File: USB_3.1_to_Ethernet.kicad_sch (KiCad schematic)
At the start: 5 parts, among them J1 RJ45_JK0654219, U1 LAN7801_9JX, U2 93LC56B_SN, U3 KSZ9031RNXCC, Y1 C3E-8.000-18-3030-R

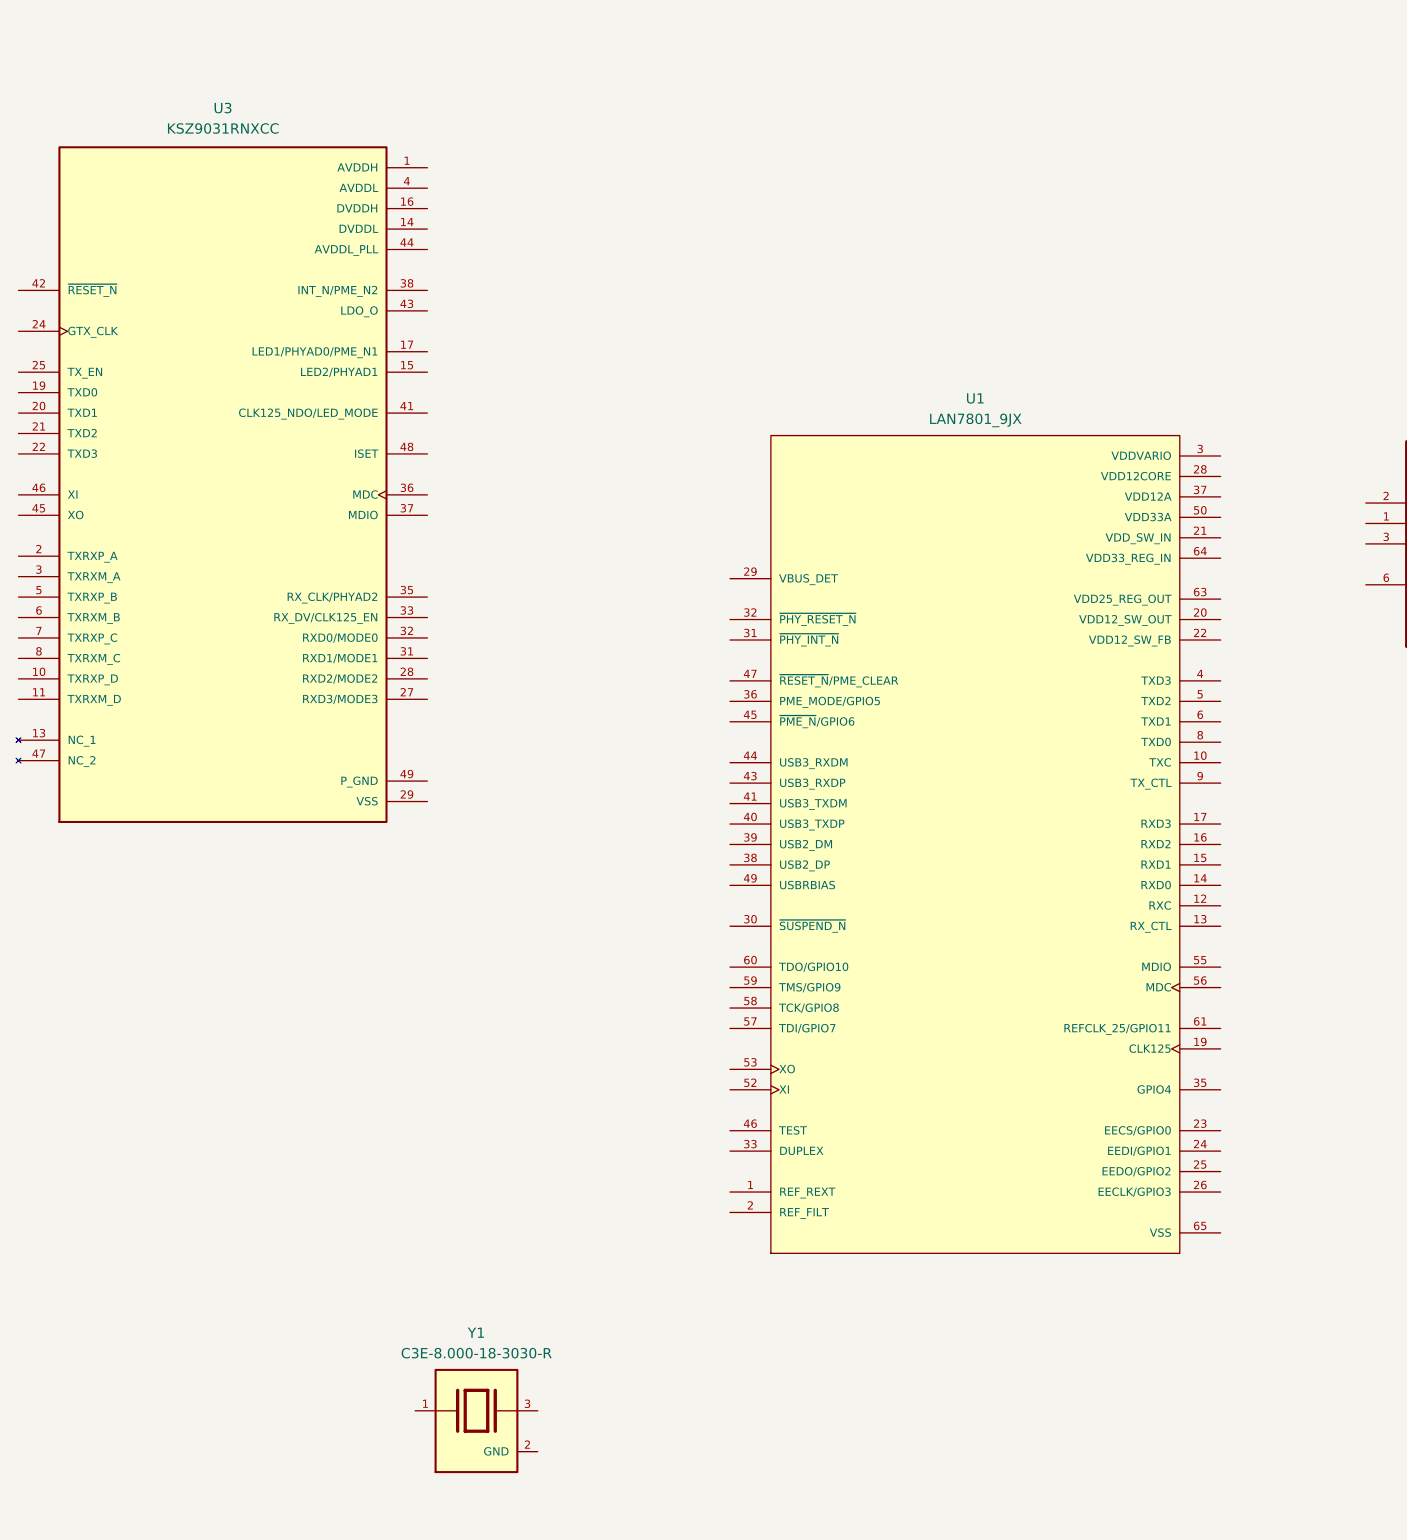
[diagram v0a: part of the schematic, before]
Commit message: power section added and power conections made
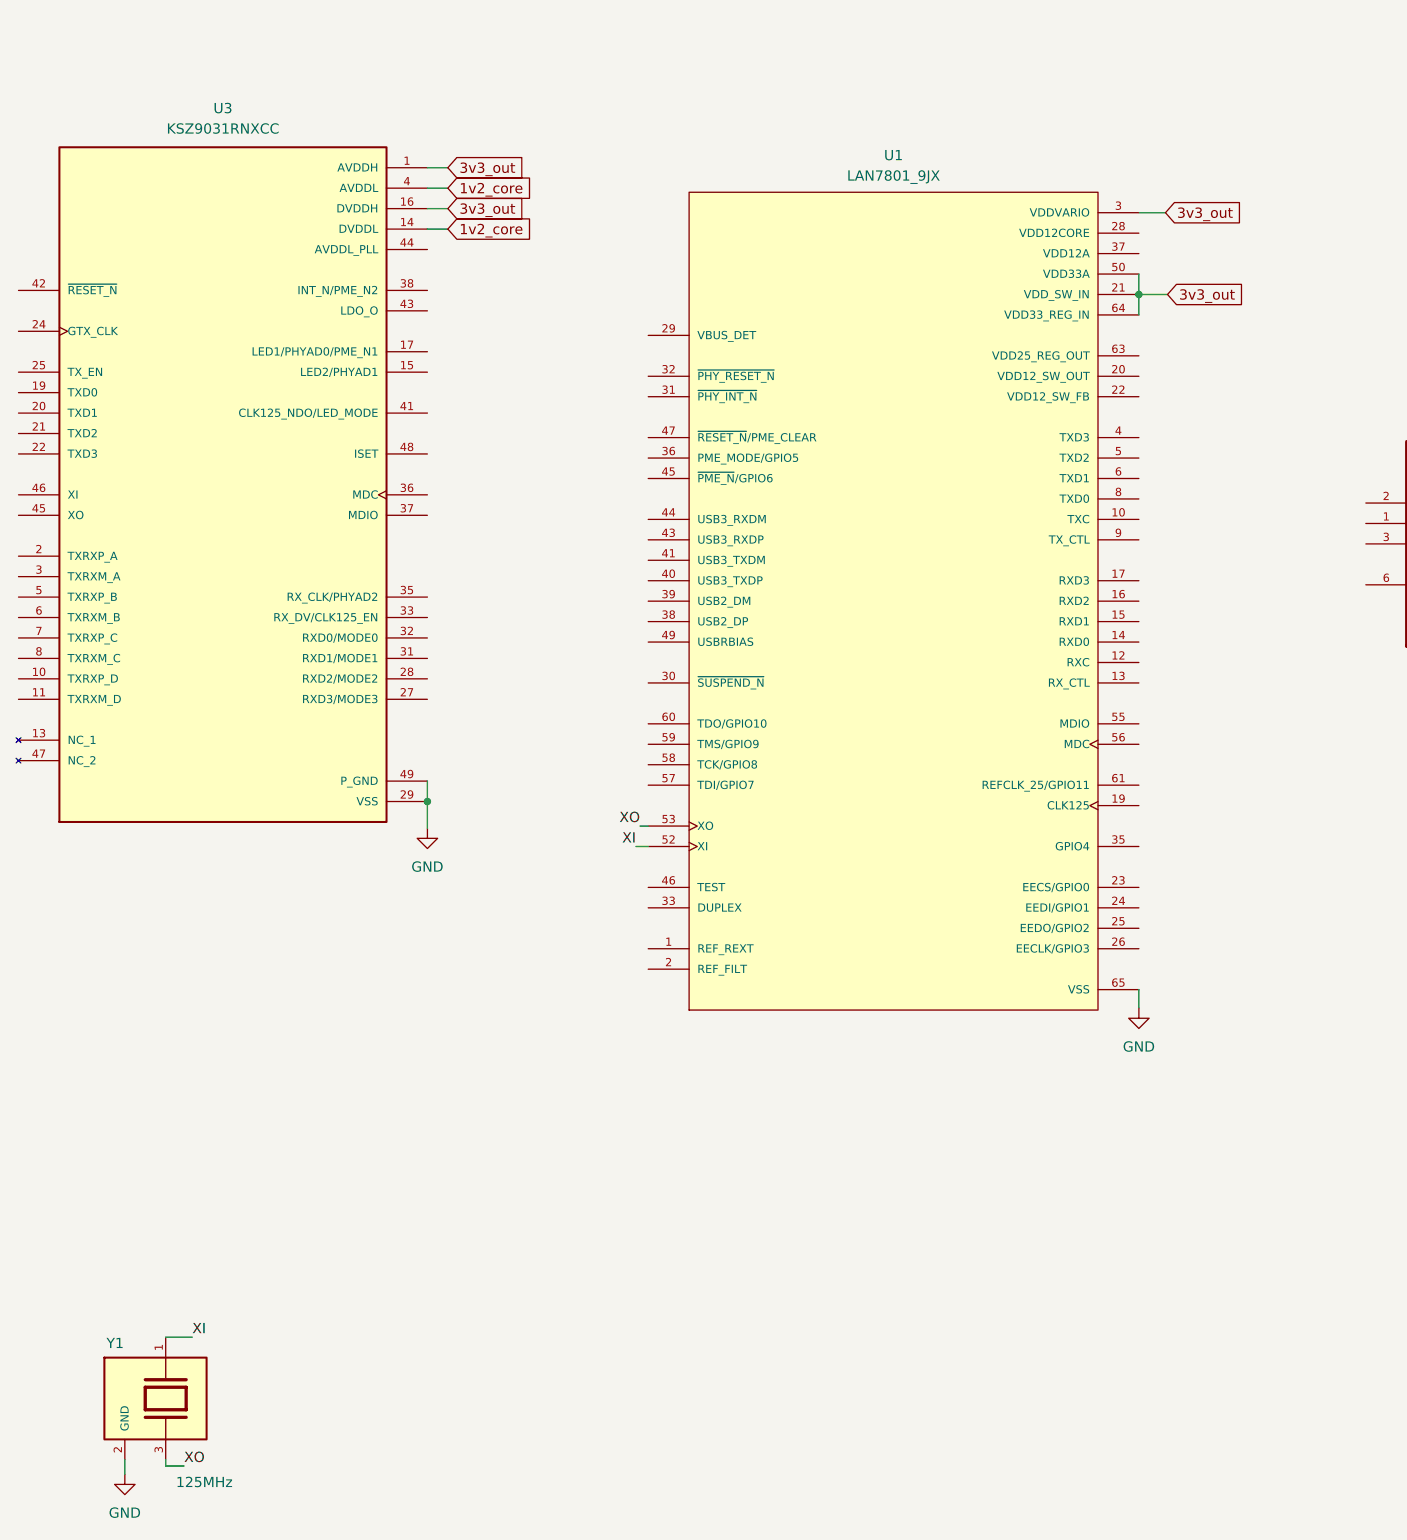
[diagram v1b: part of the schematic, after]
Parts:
- Y1: value C3E-8.000-18-3030-R -> 125MHz
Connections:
- net DVDDH is gone; now on net AVDDH: U3.16 (DVDDH), U3.34 (DVDDH), U3.40 (DVDDH)
- net DVDDL is gone; now on net AVDDL: U3.14 (DVDDL), U3.18 (DVDDL), U3.23 (DVDDL), U3.26 (DVDDL), U3.30 (DVDDL), U3.39 (DVDDL)
- net P_GND is gone; now on net GND: U3.49 (P_GND), U3.49_1 (P_GND), U3.49_10 (P_GND), U3.49_11 (P_GND), U3.49_12 (P_GND), U3.49_13 (P_GND), U3.49_14 (P_GND), U3.49_15 (P_GND), U3.49_16 (P_GND), U3.49_17 (P_GND), U3.49_18 (P_GND), U3.49_19 (P_GND), U3.49_2 (P_GND), U3.49_20 (P_GND), U3.49_21 (P_GND), U3.49_22 (P_GND), U3.49_23 (P_GND), U3.49_24 (P_GND), U3.49_25 (P_GND), U3.49_3 (P_GND), U3.49_4 (P_GND), U3.49_5 (P_GND), U3.49_6 (P_GND), U3.49_7 (P_GND), U3.49_8 (P_GND), U3.49_9 (P_GND)
- net VDDVARIO is gone; now on net AVDDH: U1.11 (VDDVARIO), U1.18 (VDDVARIO), U1.27 (VDDVARIO), U1.3 (VDDVARIO), U1.48 (VDDVARIO), U1.51 (VDDVARIO), U1.7 (VDDVARIO)
- net AVDDH: now also U1.21 (VDD_SW_IN), U1.50 (VDD33A), U1.64 (VDD33_REG_IN)
- net GND: now also U1.65 (VSS), U3.29 (VSS)
- net XI: now reaches Y1.1
- net XI: now also U1.52 (XI)
- net XO: now reaches Y1.3
- net XO: now also U1.53 (XO)
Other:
- moved on the sheet: U1, Y1
